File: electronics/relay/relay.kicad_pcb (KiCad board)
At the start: 2 copper layers, 19.3 x 45.5 mm, 11 parts, among them J1 Conn_01x05, J5 Conn_01x01_Female, J6 Conn_01x01_Female, J7 Conn_01x01_Female, K1 SANYOU_SRD_Form_C

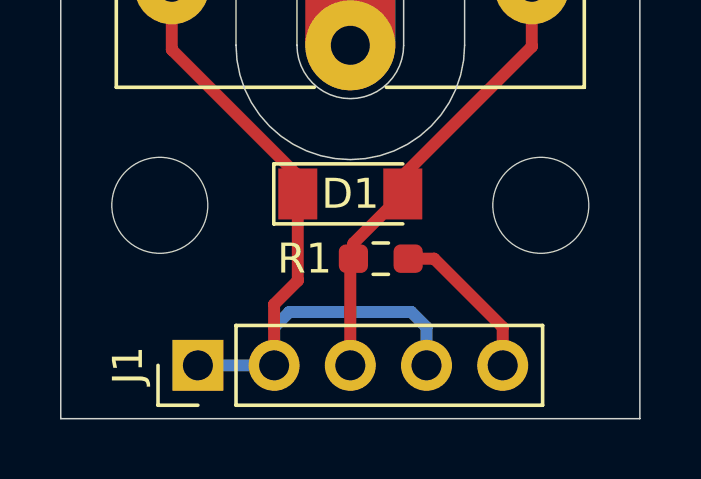
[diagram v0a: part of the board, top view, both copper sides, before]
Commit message: PCB 1st batch
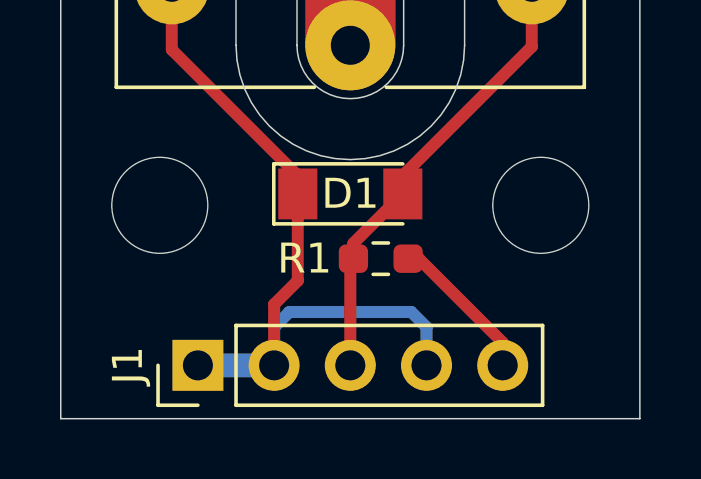
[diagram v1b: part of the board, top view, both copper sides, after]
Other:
- rule pad_to_mask_clearance: 0.051 -> 0
